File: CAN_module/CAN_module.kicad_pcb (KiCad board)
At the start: 2 copper layers, 52 parts, among them IC1 SN65HVD233QDRQ1, J2 Barrel_Jack_Switch, J4 Conn_Coaxial, J5 Screw_Terminal_01x02, U1 PC817, U2 LM5164QDDATQ1, U3 Antena BT - 2450AT42E010B001E

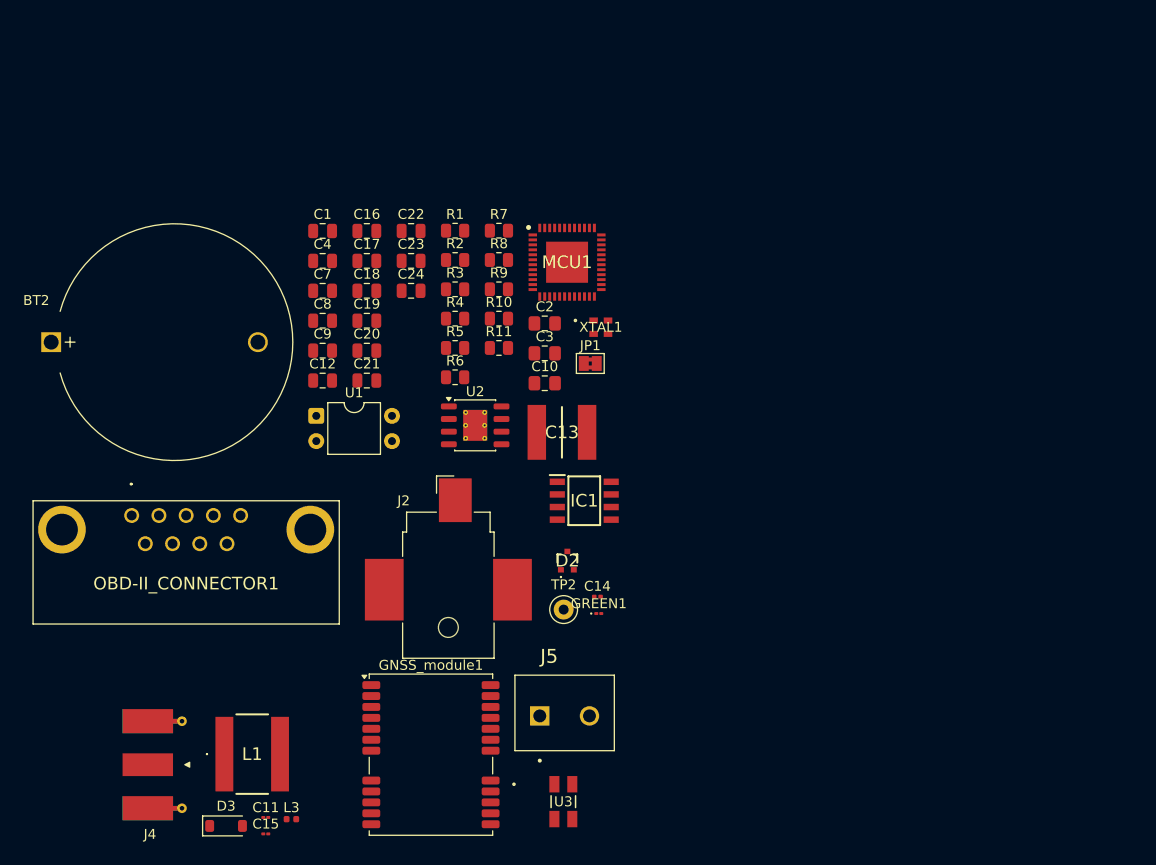
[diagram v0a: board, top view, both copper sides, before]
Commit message: Add files via upload
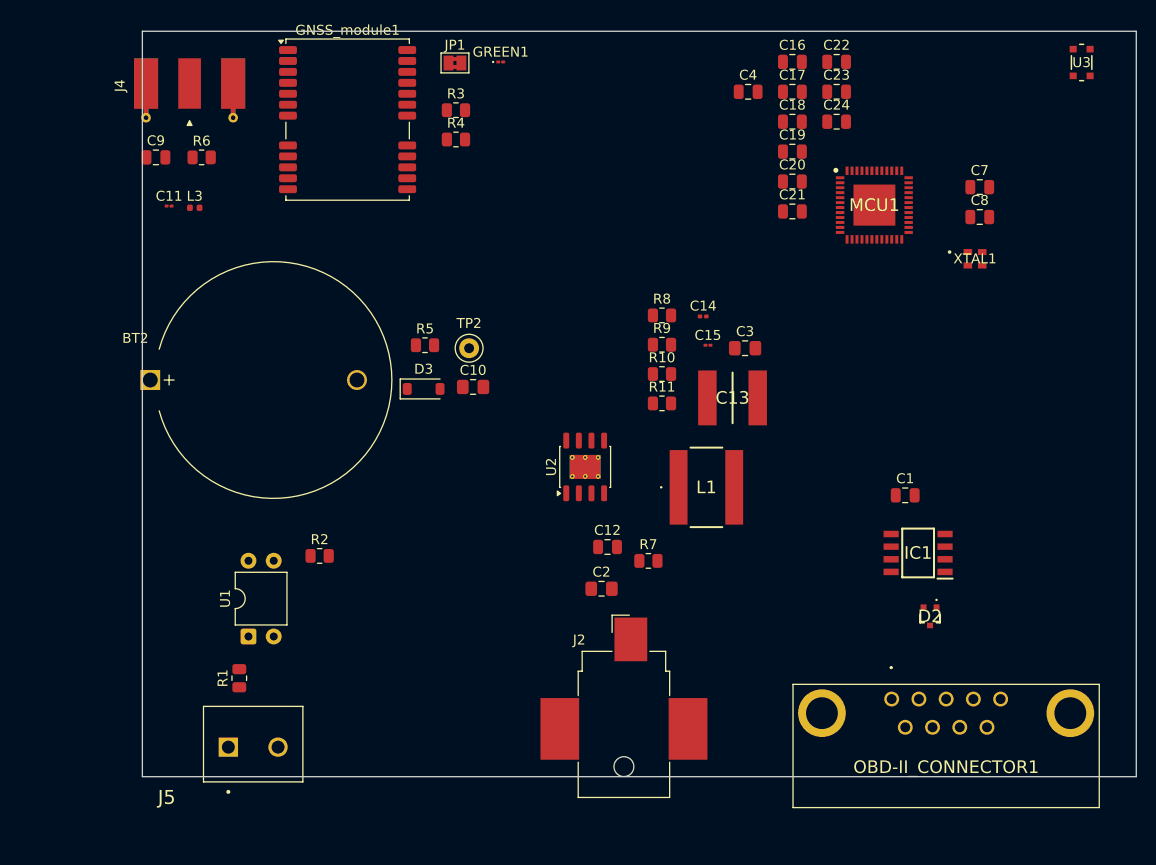
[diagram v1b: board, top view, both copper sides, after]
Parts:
- U3: value Antena BT - 2450AT42E010B001E -> Ant BT - 2450AT18D0100E; footprint Antyradar_footprints:2450AT42E010B_JOT -> Antyradar_footprints:2450AT18D0100E_JOT
- moved U3 90.8 mm to (197.2, 52.5)
- moved OBD-II_CONNECTOR1 78.7 mm to (178.0, 116.5)
- moved C7 66.9 mm to (186.9, 65.0)
- moved C8 66.9 mm to (186.9, 68.0)
- moved J4 66.9 mm to (107.4, 56.3), turned to -90 degrees
- moved C15 66.3 mm to (159.6, 80.9)
- moved GNSS_module1 64.4 mm to (123.3, 58.2)
- moved C1 64.4 mm to (179.4, 96.0)
- moved L3 62.3 mm to (107.9, 67.1)
- moved C11 62.3 mm to (105.3, 66.9)
- moved GREEN1 56.4 mm to (138.7, 52.4)
- moved L1 53.0 mm to (159.4, 95.2)
- moved R1 50.0 mm to (112.4, 114.4), turned to 90 degrees
- moved D3 48.3 mm to (130.9, 85.3)
- moved C17 46.1 mm to (168.1, 55.4)
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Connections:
- U3 pad 2: unconnected-(U3-NC-Pad2) -> GND
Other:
- board outline added: 100 x 75 mm
- copper layers 2 -> 4
